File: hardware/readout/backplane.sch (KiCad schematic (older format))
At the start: 0 parts

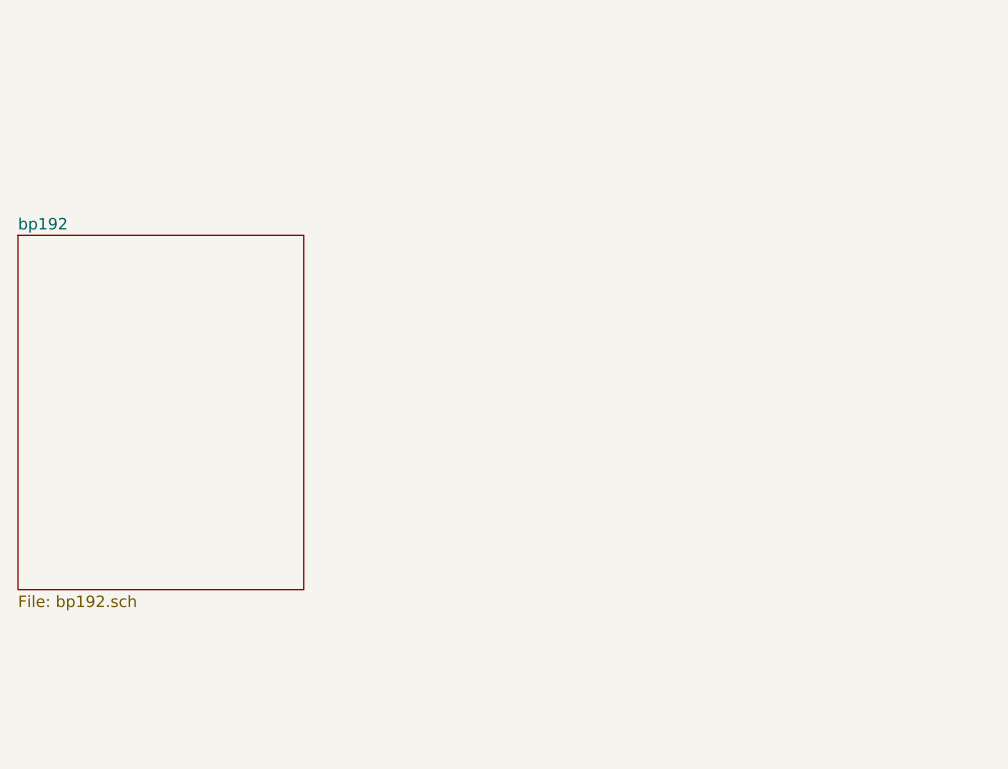
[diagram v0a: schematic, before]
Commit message: Schematic progress
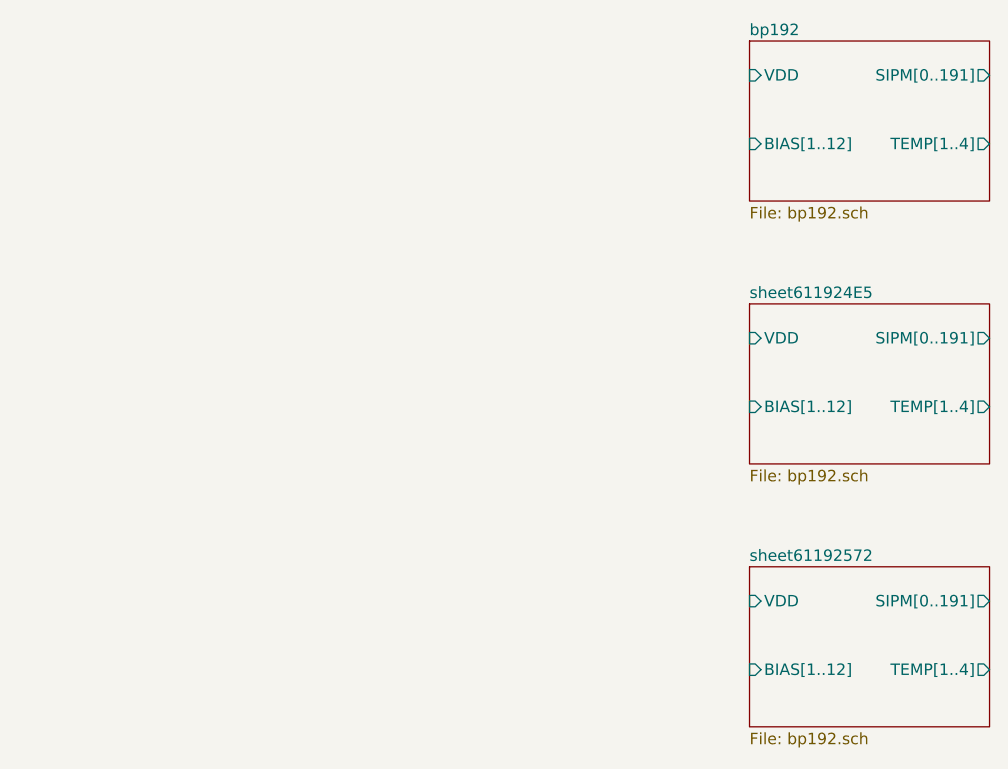
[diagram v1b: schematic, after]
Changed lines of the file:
@@
 $Descr A4 11693 8268
 encoding utf-8
-Sheet 8 9
+Sheet 8 11
 Title ""
 Date ""
@@
 $EndDescr
 $Sheet
-S 1350 2700 1250 1550
+S 4550 1850 1050 700
 U 61112853
 F0 "bp192" 50
 F1 "bp192.sch" 50
+F2 "SIPM[0..191]" O R 5600 2000 50
+F3 "VDD" I L 4550 2000 50
+F4 "BIAS[1..12]" I L 4550 2300 50
+F5 "TEMP[1..4]" O R 5600 2300 50
+$EndSheet
+$Sheet
+S 4550 3000 1050 700
+U 611924E5
+F0 "sheet611924E5" 50
+F1 "bp192.sch" 50
+F2 "SIPM[0..191]" O R 5600 3150 50
+F3 "VDD" I L 4550 3150 50
+F4 "BIAS[1..12]" I L 4550 3450 50
+F5 "TEMP[1..4]" O R 5600 3450 50
+$EndSheet
+$Sheet
+S 4550 4150 1050 700
+U 61192572
+F0 "sheet61192572" 50
+F1 "bp192.sch" 50
+F2 "SIPM[0..191]" O R 5600 4300 50
+F3 "VDD" I L 4550 4300 50
+F4 "BIAS[1..12]" I L 4550 4600 50
+F5 "TEMP[1..4]" O R 5600 4600 50
 $EndSheet
 $EndSCHEMATC
